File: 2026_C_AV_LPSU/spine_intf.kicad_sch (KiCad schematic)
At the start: 11 parts, among them IC2 LT3960EMSE#PBF, IC4 TPS7A0533PDBZR, J1 DIN41612_02x16_AB

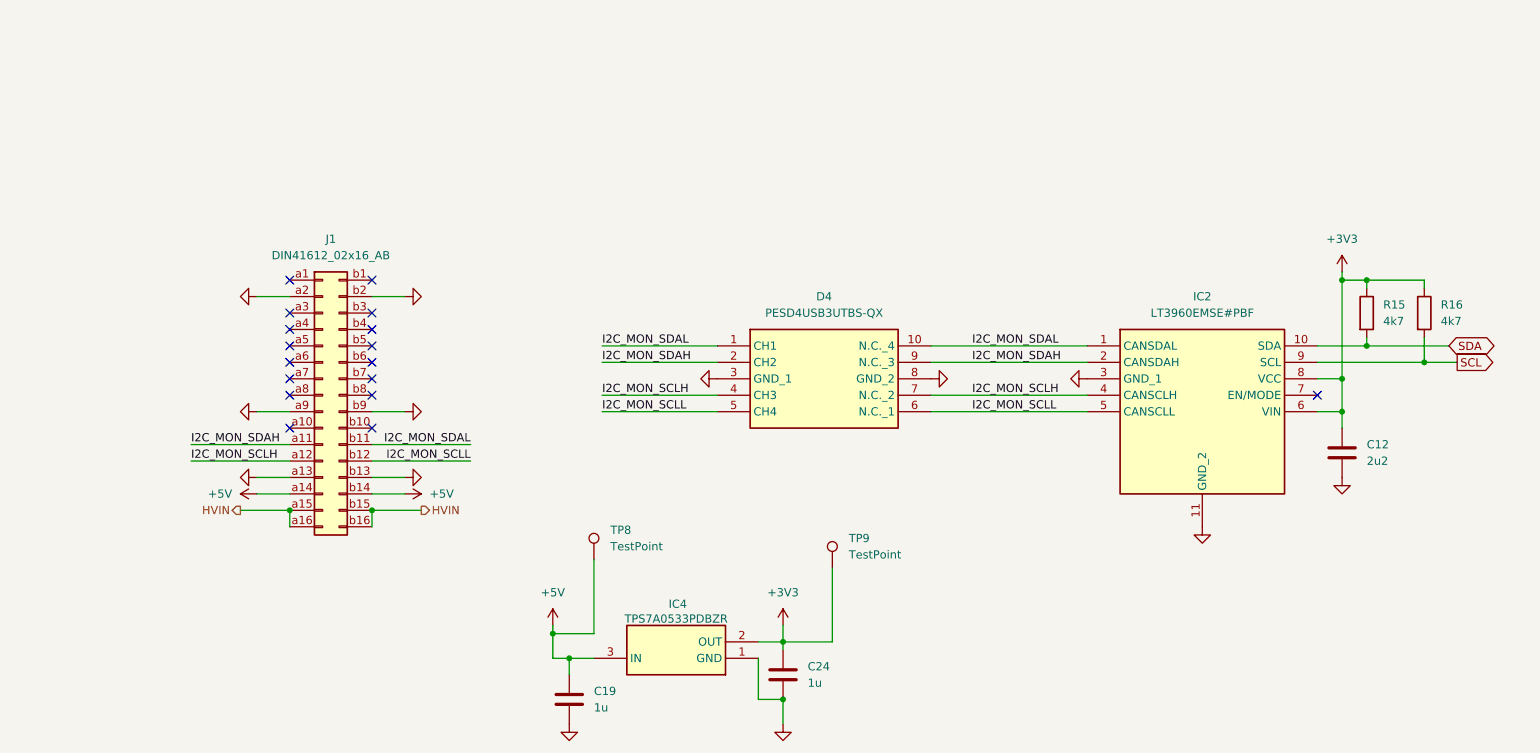
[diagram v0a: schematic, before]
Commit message: LPSU & TMB
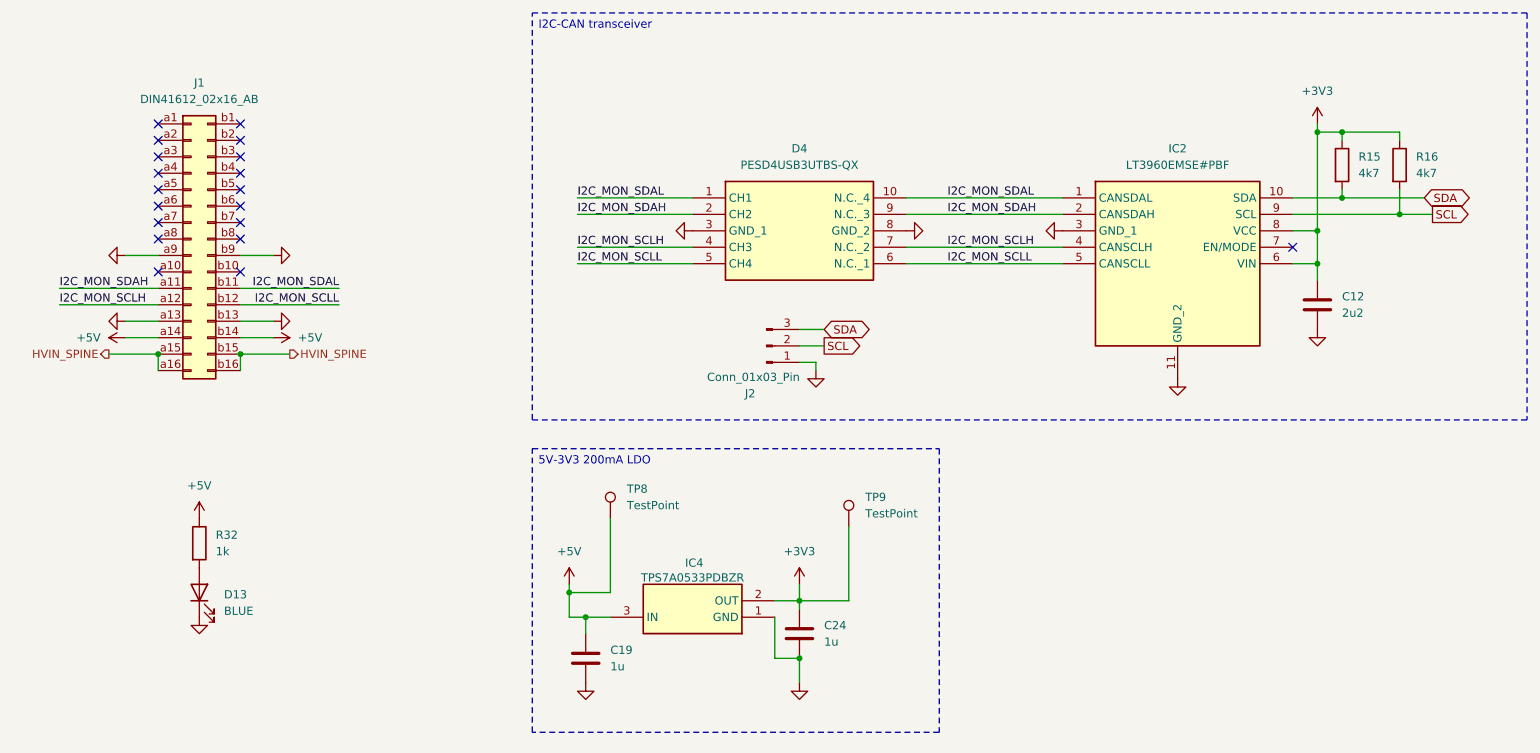
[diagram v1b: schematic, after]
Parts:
- added D13: BLUE, LED_SMD:LED_0603_1608Metric, symbol Device:LED
- added J2: Conn_01x03_Pin, Connector_PinHeader_2.54mm:PinHeader_1x03_P2.54mm_Vertical_SMD_Pin1Right, symbol Connector:Conn_01x03_Pin
- added R32: 1k, Resistor_SMD:R_0603_1608Metric, symbol Device:R
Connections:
- net +5V: now also R32.1
- net GND: now also D13.1 (K), J2.1 (Pin_1); no longer J1.a2 (Pin_a2), J1.b2 (Pin_b2)
- net SCL: now also J2.2 (Pin_2)
- net SDA: now also J2.3 (Pin_3)
- net HVIN renamed HVIN_SPINE
- new net: D13.2 (A), R32.2
- no-connect marks 17 -> 19
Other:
- company: (none) -> EPFL Rocket Team
- title: (none) -> 2026_C_AV_LPSU "ALASTOR"
- moved on the sheet: C12, C19, C24, D4, IC2, IC4, J1, R15, R16, TP8, TP9
